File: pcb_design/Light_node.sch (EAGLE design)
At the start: 39 parts, among them U10 MCP73831T-2ACI/OT, U20 LIS3DHTR, U30 ATmega328P, U40 MIC5225-3.3v, U50 COMMON_ANODE_DIODE, Y30 12MHz

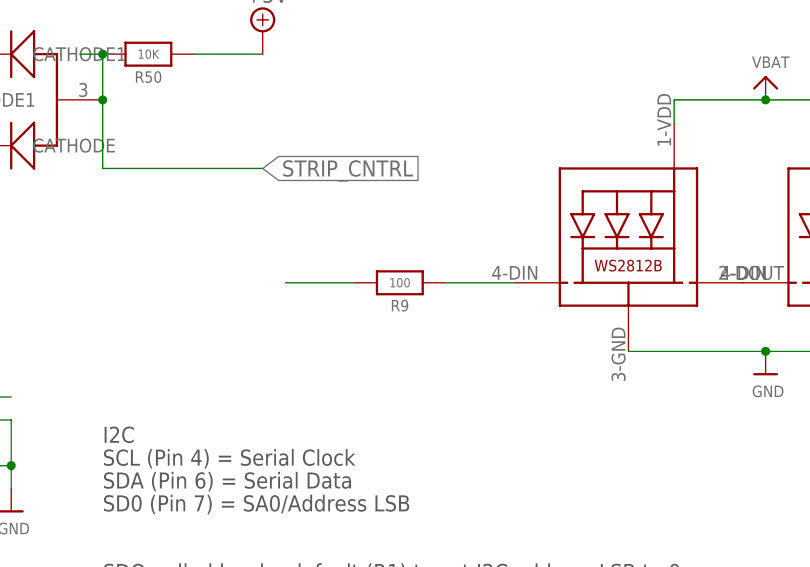
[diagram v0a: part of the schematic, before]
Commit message: got the boards running and initial code is working well!!!
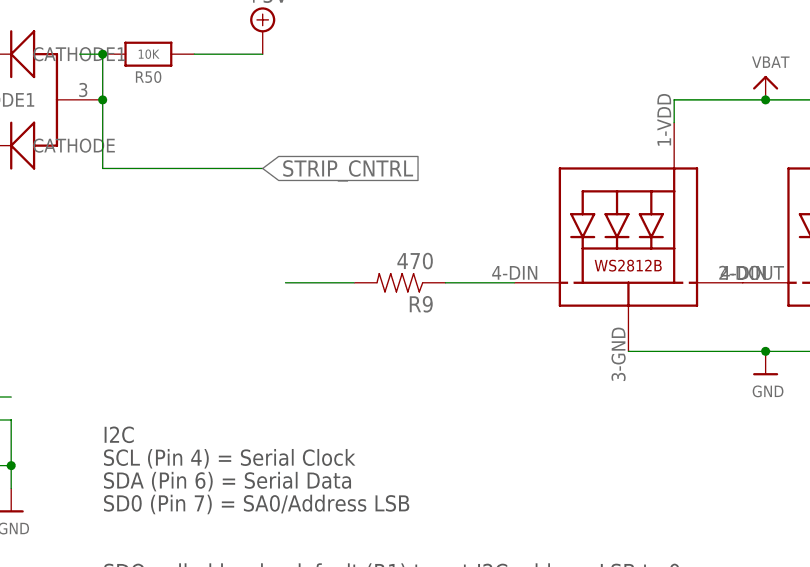
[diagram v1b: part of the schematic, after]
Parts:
- R9: value 100 -> 470; device microbuilder:RESISTOR_0603_NOOUT -> 0_shibbs2:RESISTOR0603-RES
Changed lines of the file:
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@@
 <part name="SUPPLY4" library="supply2" deviceset="+5V" device=""/>
 <part name="U$7" library="microbuilder" deviceset="VBAT" device=""/>
-<part name="R9" library="microbuilder" deviceset="RESISTOR" device="_0603_NOOUT" value="100"/>
+<part name="R9" library="0_shibbs2" deviceset="RESISTOR" device="0603-RES" value="470"/>
 <part name="U50" library="0_AlpineLabs" deviceset="COMMON_ANODE_DIODE" device=""/>
 <part name="SUPPLY5" library="supply2" deviceset="+5V" device=""/>
